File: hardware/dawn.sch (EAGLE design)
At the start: 33 parts, among them IC1 ATMEGA328-20P, IC3 DS1307, Q2 16Mhz, Q3 32.768kHz, Q4 BUZ11BV, T3 BC547B, T4 BC547B, X1 MKDSN1,5/2-5,08, X2 MKDSN1,5/2-5,08

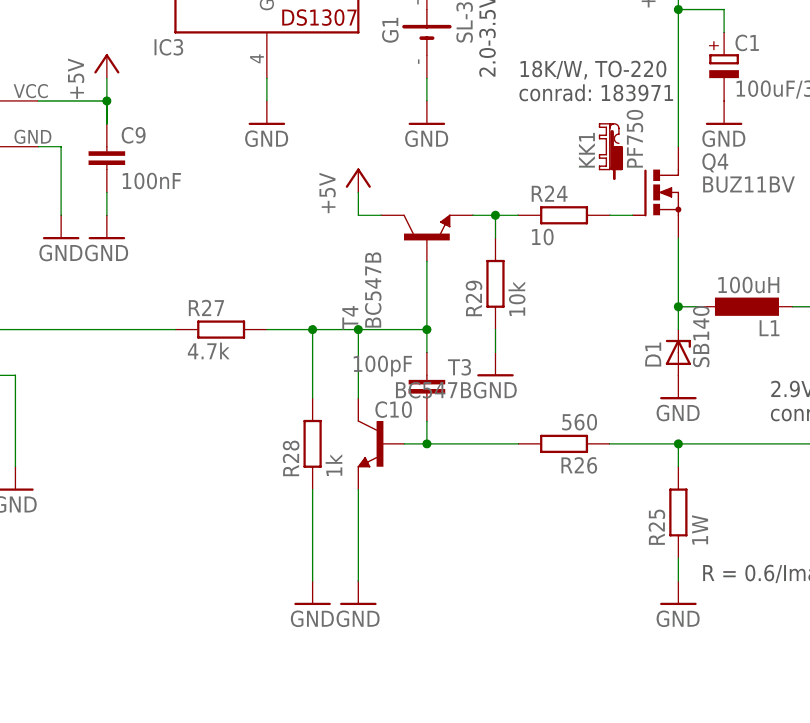
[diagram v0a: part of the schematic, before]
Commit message: Cleanup
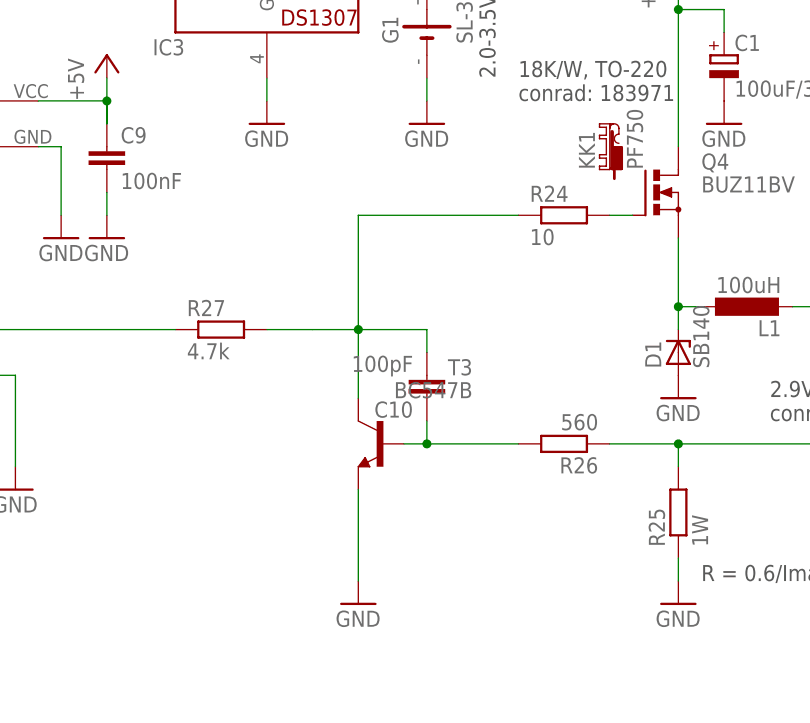
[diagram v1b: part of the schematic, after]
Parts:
- removed R28: 1k, rcl:R-EU_0204/5
- removed R29: 10k, rcl:R-EU_0204/2V
- removed T4: BC547B, transistor-neu-to92:-NPN-TO92-EBC
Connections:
- removed net N$43: R24.1, R29.2, T4.E
- net +5V: no longer T4.C
- net GND: no longer R28.1, R29.1
- net N$41: now also R24.1; no longer R28.2, T4.B
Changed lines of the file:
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@@
 <part name="GND25" library="supply1" deviceset="GND" device=""/>
 <part name="R27" library="rcl" deviceset="R-EU_" device="0207/10" value="4.7k"/>
-<part name="R28" library="rcl" deviceset="R-EU_" device="0204/5" value="1k"/>
-<part name="GND26" library="supply1" deviceset="GND" device=""/>
-<part name="T4" library="transistor-neu-to92" deviceset="*-NPN-" device="TO92-EBC" value="BC547B"/>
-<part name="R29" library="rcl" deviceset="R-EU_" device="0204/2V" value="10k"/>
-<part name="GND27" library="supply1" deviceset="GND" device=""/>
-<part name="P+1" library="supply1" deviceset="+5V" device=""/>
 <part name="P+2" library="supply1" deviceset="+5V" device=""/>
 <part name="X1" library="con-phoenix-508" deviceset="MKDSN1,5/2-5,08" device=""/>
@@
 <instance part="GND25" gate="1" x="93.98" y="-83.82"/>
 <instance part="R27" gate="G$1" x="78.74" y="-53.34"/>
-<instance part="R28" gate="G$1" x="88.9" y="-66.04" rot="R90"/>
-<instance part="GND26" gate="1" x="88.9" y="-83.82"/>
-<instance part="T4" gate="G$1" x="101.6" y="-43.18" rot="R90"/>
-<instance part="R29" gate="G$1" x="109.22" y="-48.26" rot="R90"/>
-<instance part="GND27" gate="1" x="109.22" y="-58.42"/>
-<instance part="P+1" gate="1" x="93.98" y="-35.56"/>
 <instance part="P+2" gate="1" x="129.54" y="-12.7"/>
 <instance part="X1" gate="-1" x="149.86" y="2.54"/>
@@
 </segment>
 <segment>
-<pinref part="T4" gate="G$1" pin="C"/>
-<wire x1="93.98" y1="-38.1" x2="93.98" y2="-40.64" width="0.1524" layer="91"/>
-<wire x1="93.98" y1="-40.64" x2="96.52" y2="-40.64" width="0.1524" layer="91"/>
-<pinref part="P+1" gate="1" pin="+5V"/>
-</segment>
-<segment>
 <pinref part="P+12" gate="1" pin="+5V"/>
 <wire x1="144.78" y1="7.62" x2="144.78" y2="10.16" width="0.1524" layer="91"/>
@@
 <pinref part="GND24" gate="1" pin="GND"/>
 <wire x1="129.54" y1="-78.74" x2="129.54" y2="-81.28" width="0.1524" layer="91"/>
-</segment>
-<segment>
-<pinref part="R28" gate="G$1" pin="1"/>
-<pinref part="GND26" gate="1" pin="GND"/>
-<wire x1="88.9" y1="-81.28" x2="88.9" y2="-71.12" width="0.1524" layer="91"/>
-</segment>
-<segment>
-<pinref part="R29" gate="G$1" pin="1"/>
-<pinref part="GND27" gate="1" pin="GND"/>
-<wire x1="109.22" y1="-55.88" x2="109.22" y2="-53.34" width="0.1524" layer="91"/>
 </segment>
 <segment>
@@
 <wire x1="101.6" y1="-53.34" x2="93.98" y2="-53.34" width="0.1524" layer="91"/>
 <wire x1="93.98" y1="-53.34" x2="93.98" y2="-60.96" width="0.1524" layer="91"/>
-<pinref part="T4" gate="G$1" pin="B"/>
-<wire x1="101.6" y1="-45.72" x2="101.6" y2="-53.34" width="0.1524" layer="91"/>
-<junction x="101.6" y="-53.34"/>
-<pinref part="R28" gate="G$1" pin="2"/>
-<wire x1="88.9" y1="-53.34" x2="88.9" y2="-60.96" width="0.1524" layer="91"/>
 <wire x1="88.9" y1="-53.34" x2="83.82" y2="-53.34" width="0.1524" layer="91"/>
 <wire x1="93.98" y1="-53.34" x2="88.9" y2="-53.34" width="0.1524" layer="91"/>
 <pinref part="R27" gate="G$1" pin="2"/>
-<junction x="88.9" y="-53.34"/>
 <junction x="93.98" y="-53.34"/>
-</segment>
-</net>
-<net name="N$43" class="0">
-<segment>
 <pinref part="R24" gate="G$1" pin="1"/>
-<pinref part="R29" gate="G$1" pin="2"/>
-<wire x1="111.76" y1="-40.64" x2="109.22" y2="-40.64" width="0.1524" layer="91"/>
-<wire x1="109.22" y1="-40.64" x2="109.22" y2="-43.18" width="0.1524" layer="91"/>
-<pinref part="T4" gate="G$1" pin="E"/>
-<wire x1="109.22" y1="-40.64" x2="106.68" y2="-40.64" width="0.1524" layer="91"/>
-<junction x="109.22" y="-40.64"/>
-</segment>
-</net>
+<wire x1="111.76" y1="-40.64" x2="93.98" y2="-40.64" width="0.1524" layer="91"/>
+<wire x1="93.98" y1="-40.64" x2="93.98" y2="-53.34" width="0.1524" layer="91"/>
+</segment>
+</net>

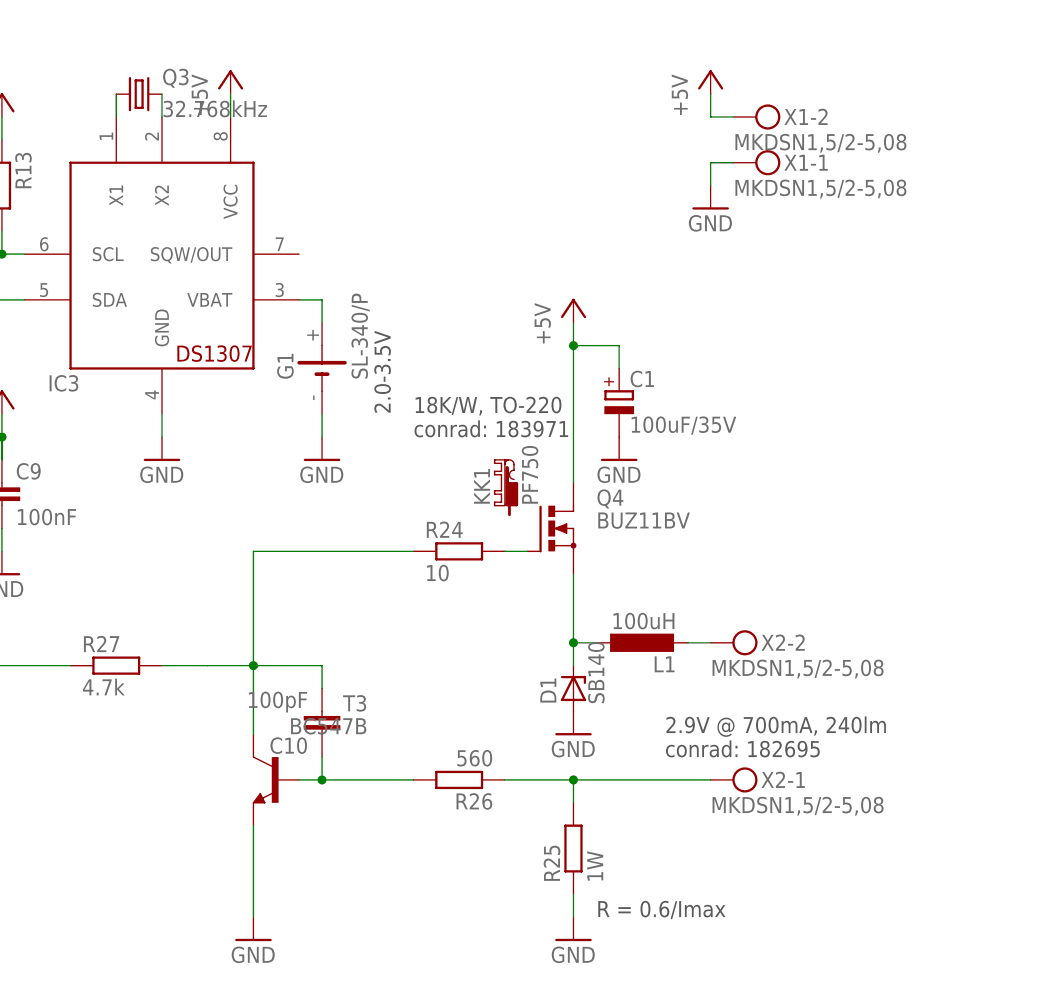
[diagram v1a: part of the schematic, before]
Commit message: Fixed minors.
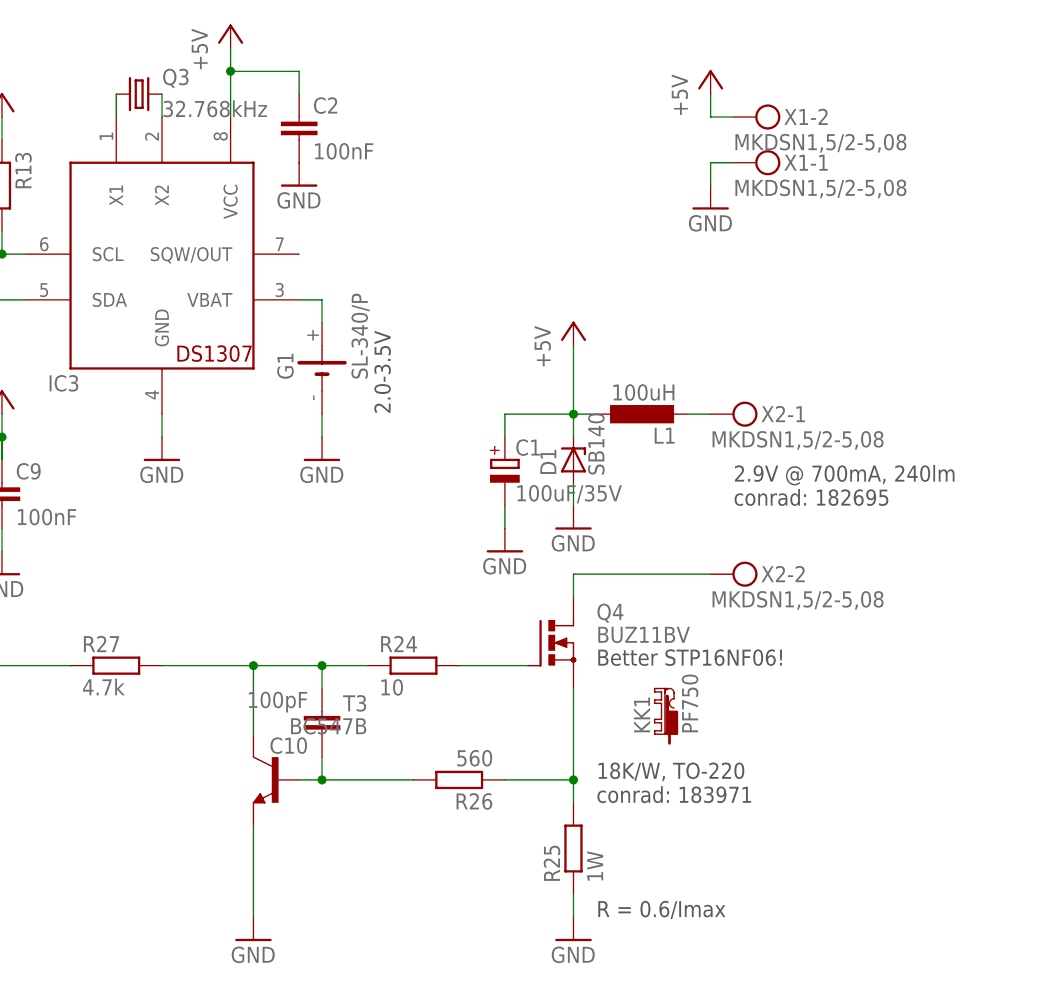
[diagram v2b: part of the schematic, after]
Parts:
- added C2: 100nF, rcl:C-EU025-025X050
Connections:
- removed net N$15: L1.2, X2-2.KL
- new net N$16: Q4.D, X2-2.KL
- net +5V: now also C2.1, D1.C, L1.1; no longer Q4.D
- net GND: now also C2.2
- net N$11: now also L1.2, X2-1.KL; no longer D1.C, L1.1, Q4.S
- net N$39: now also Q4.S; no longer X2-1.KL
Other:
- note added: "Better STP16NF06!"
- moved on the sheet: C1, D1, KK1, L1, Q4, R24, X2-1, X2-2
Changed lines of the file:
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@@
 <?xml version="1.0" encoding="utf-8"?>
 <!DOCTYPE eagle SYSTEM "eagle.dtd">
-<eagle version="7.1.0">
+<eagle version="7.5.0">
 <drawing>
 <settings>
@@
 <part name="GND8" library="supply1" deviceset="GND" device=""/>
 <part name="U$2" library="isp" deviceset="AVR-ISP" device=""/>
+<part name="C2" library="rcl" deviceset="C-EU" device="025-025X050" value="100nF"/>
+<part name="GND7" library="supply1" deviceset="GND" device=""/>
 </parts>
 <sheets>
 <sheet>
 <plain>
-<text x="139.7" y="-63.5" size="1.778" layer="97">2.9V @ 700mA, 240lm
+<text x="147.32" y="-35.56" size="1.778" layer="97">2.9V @ 700mA, 240lm
 conrad: 182695</text>
-<text x="111.76" y="-27.94" size="1.778" layer="97">18K/W, TO-220
+<text x="132.08" y="-68.58" size="1.778" layer="97">18K/W, TO-220
 conrad: 183971</text>
 <text x="109.22" y="-25.4" size="1.778" layer="97" rot="R90">2.0-3.5V</text>
 <text x="132.08" y="-81.28" size="1.778" layer="97">R = 0.6/Imax</text>
+<text x="132.08" y="-53.34" size="1.778" layer="97">Better STP16NF06!</text>
 </plain>
 <instances>
@@
 <instance part="GND16" gate="1" x="-43.18" y="-53.34"/>
 <instance part="GND15" gate="1" x="83.82" y="-30.48"/>
-<instance part="P+8" gate="1" x="91.44" y="12.7"/>
+<instance part="P+8" gate="1" x="91.44" y="17.78"/>
 <instance part="G1" gate="G$1" x="101.6" y="-20.32" rot="R90"/>
 <instance part="GND17" gate="1" x="101.6" y="-30.48"/>
@@
 <instance part="P+12" gate="1" x="144.78" y="12.7"/>
 <instance part="GND20" gate="1" x="144.78" y="-2.54"/>
-<instance part="R24" gate="G$1" x="116.84" y="-40.64"/>
-<instance part="Q4" gate="1" x="127" y="-38.1"/>
+<instance part="R24" gate="G$1" x="111.76" y="-53.34"/>
+<instance part="Q4" gate="1" x="127" y="-50.8"/>
 <instance part="R25" gate="G$1" x="129.54" y="-73.66" rot="R90"/>
 <instance part="R26" gate="G$1" x="116.84" y="-66.04" rot="R180"/>
@@
 <instance part="GND25" gate="1" x="93.98" y="-83.82"/>
 <instance part="R27" gate="G$1" x="78.74" y="-53.34"/>
-<instance part="P+2" gate="1" x="129.54" y="-12.7"/>
+<instance part="P+2" gate="1" x="129.54" y="-15.24"/>
 <instance part="X1" gate="-1" x="149.86" y="2.54"/>
 <instance part="X1" gate="-2" x="149.86" y="7.62"/>
-<instance part="X2" gate="-1" x="147.32" y="-66.04"/>
-<instance part="X2" gate="-2" x="147.32" y="-50.8"/>
+<instance part="X2" gate="-1" x="147.32" y="-25.4"/>
+<instance part="X2" gate="-2" x="147.32" y="-43.18"/>
 <instance part="IC1" gate="G$1" x="-12.7" y="-30.48"/>
 <instance part="GND2" gate="1" x="-10.16" y="-91.44"/>
@@
 <instance part="JP1" gate="A" x="43.18" y="-68.58" rot="R270"/>
 <instance part="GND5" gate="1" x="55.88" y="-71.12"/>
-<instance part="KK1" gate="G$1" x="121.92" y="-33.02"/>
+<instance part="KK1" gate="G$1" x="139.7" y="-58.42"/>
 <instance part="R1" gate="G$1" x="35.56" y="-2.54"/>
 <instance part="R2" gate="1" x="22.86" y="5.08"/>
 <instance part="P+5" gate="1" x="22.86" y="15.24"/>
 <instance part="GND6" gate="1" x="43.18" y="-7.62"/>
-<instance part="L1" gate="G$1" x="137.16" y="-50.8" rot="R90"/>
-<instance part="C1" gate="G$1" x="134.62" y="-22.86"/>
-<instance part="D1" gate="G$1" x="129.54" y="-55.88" rot="R90"/>
-<instance part="GND1" gate="1" x="134.62" y="-30.48"/>
-<instance part="GND8" gate="1" x="129.54" y="-60.96"/>
+<instance part="L1" gate="G$1" x="137.16" y="-25.4" rot="R90"/>
+<instance part="C1" gate="G$1" x="121.92" y="-30.48"/>
+<instance part="D1" gate="G$1" x="129.54" y="-30.48" rot="R90"/>
+<instance part="GND1" gate="1" x="121.92" y="-40.64"/>
+<instance part="GND8" gate="1" x="129.54" y="-38.1"/>
 <instance part="U$2" gate="G$1" x="7.62" y="-81.28" rot="MR0"/>
+<instance part="C2" gate="G$1" x="99.06" y="7.62"/>
+<instance part="GND7" gate="1" x="99.06" y="0"/>
 </instances>
 <busses>
@@
 <pinref part="P+8" gate="1" pin="+5V"/>
 <pinref part="IC3" gate="G$1" pin="VCC"/>
-<wire x1="91.44" y1="10.16" x2="91.44" y2="7.62" width="0.1524" layer="91"/>
+<wire x1="91.44" y1="15.24" x2="91.44" y2="12.7" width="0.1524" layer="91"/>
+<pinref part="C2" gate="G$1" pin="1"/>
+<wire x1="91.44" y1="12.7" x2="91.44" y2="7.62" width="0.1524" layer="91"/>
+<wire x1="99.06" y1="10.16" x2="99.06" y2="12.7" width="0.1524" layer="91"/>
+<wire x1="99.06" y1="12.7" x2="91.44" y2="12.7" width="0.1524" layer="91"/>
+<junction x="91.44" y="12.7"/>
 </segment>
 <segment>
@@
 <segment>
 <pinref part="P+2" gate="1" pin="+5V"/>
-<pinref part="Q4" gate="1" pin="D"/>
-<wire x1="129.54" y1="-15.24" x2="129.54" y2="-17.78" width="0.1524" layer="91"/>
-<wire x1="129.54" y1="-17.78" x2="129.54" y2="-33.02" width="0.1524" layer="91"/>
-<wire x1="129.54" y1="-17.78" x2="134.62" y2="-17.78" width="0.1524" layer="91"/>
+<wire x1="129.54" y1="-17.78" x2="129.54" y2="-25.4" width="0.1524" layer="91"/>
+<wire x1="129.54" y1="-25.4" x2="121.92" y2="-25.4" width="0.1524" layer="91"/>
 <pinref part="C1" gate="G$1" pin="+"/>
-<wire x1="134.62" y1="-17.78" x2="134.62" y2="-20.32" width="0.1524" layer="91"/>
-<junction x="129.54" y="-17.78"/>
+<wire x1="121.92" y1="-25.4" x2="121.92" y2="-27.94" width="0.1524" layer="91"/>
+<pinref part="D1" gate="G$1" pin="C"/>
+<pinref part="L1" gate="G$1" pin="1"/>
+<wire x1="129.54" y1="-25.4" x2="129.54" y2="-27.94" width="0.1524" layer="91"/>
+<wire x1="129.54" y1="-25.4" x2="132.08" y2="-25.4" width="0.1524" layer="91"/>
+<junction x="129.54" y="-25.4"/>
 </segment>
 </net>
@@
 <pinref part="C1" gate="G$1" pin="-"/>
 <pinref part="GND1" gate="1" pin="GND"/>
+<wire x1="121.92" y1="-35.56" x2="121.92" y2="-38.1" width="0.1524" layer="91"/>
 </segment>
 <segment>
 <pinref part="D1" gate="G$1" pin="A"/>
 <pinref part="GND8" gate="1" pin="GND"/>
+<wire x1="129.54" y1="-33.02" x2="129.54" y2="-35.56" width="0.1524" layer="91"/>
+</segment>
+<segment>
+<pinref part="C2" gate="G$1" pin="2"/>
+<pinref part="GND7" gate="1" pin="GND"/>
 </segment>
 </net>
@@
 <pinref part="Q4" gate="1" pin="G"/>
 <pinref part="R24" gate="G$1" pin="2"/>
-<wire x1="121.92" y1="-40.64" x2="124.46" y2="-40.64" width="0.1524" layer="91"/>
+<wire x1="116.84" y1="-53.34" x2="124.46" y2="-53.34" width="0.1524" layer="91"/>
 </segment>
 </net>
@@
 <wire x1="121.92" y1="-66.04" x2="129.54" y2="-66.04" width="0.1524" layer="91"/>
 <junction x="129.54" y="-66.04"/>
-<wire x1="129.54" y1="-66.04" x2="144.78" y2="-66.04" width="0.1524" layer="91"/>
-<pinref part="X2" gate="-1" pin="KL"/>
+<pinref part="Q4" gate="1" pin="S"/>
+<wire x1="129.54" y1="-55.88" x2="129.54" y2="-66.04" width="0.1524" layer="91"/>
 </segment>
 </net>
@@
 <wire x1="101.6" y1="-53.34" x2="101.6" y2="-55.88" width="0.1524" layer="91"/>
 <pinref part="T3" gate="G$1" pin="C"/>
-<wire x1="101.6" y1="-53.34" x2="93.98" y2="-53.34" width="0.1524" layer="91"/>
 <wire x1="93.98" y1="-53.34" x2="93.98" y2="-60.96" width="0.1524" layer="91"/>
-<wire x1="88.9" y1="-53.34" x2="83.82" y2="-53.34" width="0.1524" layer="91"/>
-<wire x1="93.98" y1="-53.34" x2="88.9" y2="-53.34" width="0.1524" layer="91"/>
+<wire x1="93.98" y1="-53.34" x2="83.82" y2="-53.34" width="0.1524" layer="91"/>
 <pinref part="R27" gate="G$1" pin="2"/>
 <junction x="93.98" y="-53.34"/>
 <pinref part="R24" gate="G$1" pin="1"/>
-<wire x1="111.76" y1="-40.64" x2="93.98" y2="-40.64" width="0.1524" layer="91"/>
-<wire x1="93.98" y1="-40.64" x2="93.98" y2="-53.34" width="0.1524" layer="91"/>
+<wire x1="106.68" y1="-53.34" x2="101.6" y2="-53.34" width="0.1524" layer="91"/>
+<wire x1="101.6" y1="-53.34" x2="93.98" y2="-53.34" width="0.1524" layer="91"/>
+<junction x="101.6" y="-53.34"/>
 </segment>
 </net>
@@
 </segment>
 </net>
+<net name="N$16" class="0">
+<segment>
+<pinref part="Q4" gate="1" pin="D"/>
+<wire x1="129.54" y1="-43.18" x2="129.54" y2="-45.72" width="0.1524" layer="91"/>
+<pinref part="X2" gate="-2" pin="KL"/>
+<wire x1="144.78" y1="-43.18" x2="129.54" y2="-43.18" width="0.1524" layer="91"/>
+</segment>
+</net>
 <net name="N$11" class="0">
 <segment>
-<pinref part="Q4" gate="1" pin="S"/>
-<pinref part="D1" gate="G$1" pin="C"/>
-<wire x1="129.54" y1="-43.18" x2="129.54" y2="-50.8" width="0.1524" layer="91"/>
-<pinref part="L1" gate="G$1" pin="1"/>
-<wire x1="129.54" y1="-50.8" x2="129.54" y2="-53.34" width="0.1524" layer="91"/>
-<wire x1="129.54" y1="-50.8" x2="132.08" y2="-50.8" width="0.1524" layer="91"/>
-<junction x="129.54" y="-50.8"/>
-</segment>
-</net>
-<net name="N$15" class="0">
-<segment>
 <pinref part="L1" gate="G$1" pin="2"/>
-<pinref part="X2" gate="-2" pin="KL"/>
-<wire x1="142.24" y1="-50.8" x2="144.78" y2="-50.8" width="0.1524" layer="91"/>
-</segment>
-</net>
+<pinref part="X2" gate="-1" pin="KL"/>
+<wire x1="142.24" y1="-25.4" x2="144.78" y2="-25.4" width="0.1524" layer="91"/>
+</segment>
+</net>
